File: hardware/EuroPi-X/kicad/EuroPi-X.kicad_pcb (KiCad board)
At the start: 2 copper layers, 86.5 x 109.2 mm, 154 parts, among them J1 Conn_01x16_Pin, J10 Thonkiconn_Mono_Jack, J11 Conn_02x08_Odd_Even, J12 Thonkiconn_Mono_Jack, J13 Thonkiconn_Mono_Jack, J14 Thonkiconn_Mono_Jack, J15 Thonkiconn_Mono_Jack, J16 Thonkiconn_Mono_Jack, J17 Thonkiconn_Mono_Jack, J18 Conn_01x30_Pin, J19 Conn_01x04_Pin, J2 Conn_01x16_Pin, J20 Conn_01x04_Pin, J21 Conn_01x04_Pin, J3 Thonkiconn_Mono_Jack, J4 Thonkiconn_Mono_Jack, J5 Conn_01x16_Pin, J6 Thonkiconn_Mono_Jack, J7 Thonkiconn_Mono_Jack, J8 Conn_01x16_Pin, J9 Thonkiconn_Mono_Jack, P1 USB_C_Plug_USB2.0, P2 Potentiometer_9mm_Vertical_Li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, P3 Potentiometer_9mm_Vertical_Li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, SW1 B1, SW2 B2, U1 LM4030-4.096, U10 MCP3428, U11 L7805, U2 LM4040DBZ-2.0, U3 LM4040DBZ-10, U4 RP2040, U7 TL074, U8 TL074, U9 MCP6004, Y1 Crystal_GND2

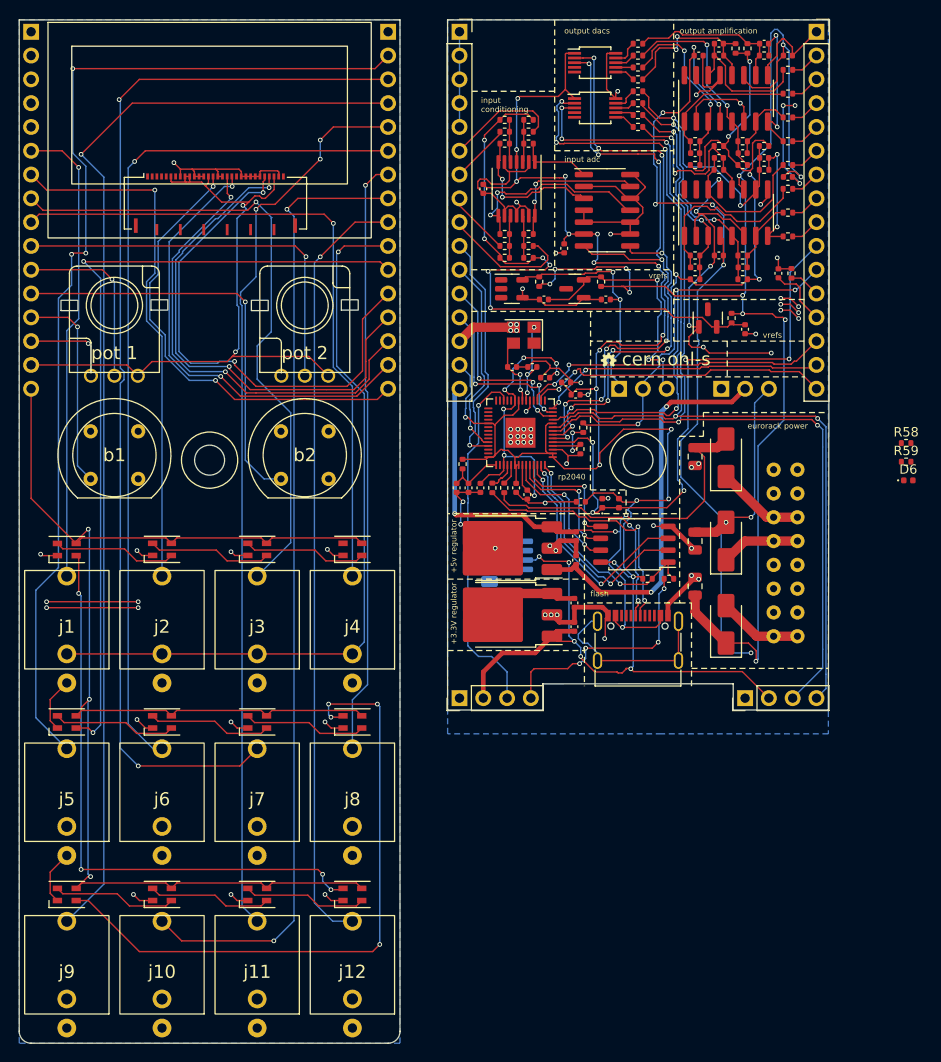
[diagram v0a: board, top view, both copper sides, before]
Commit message: save and export
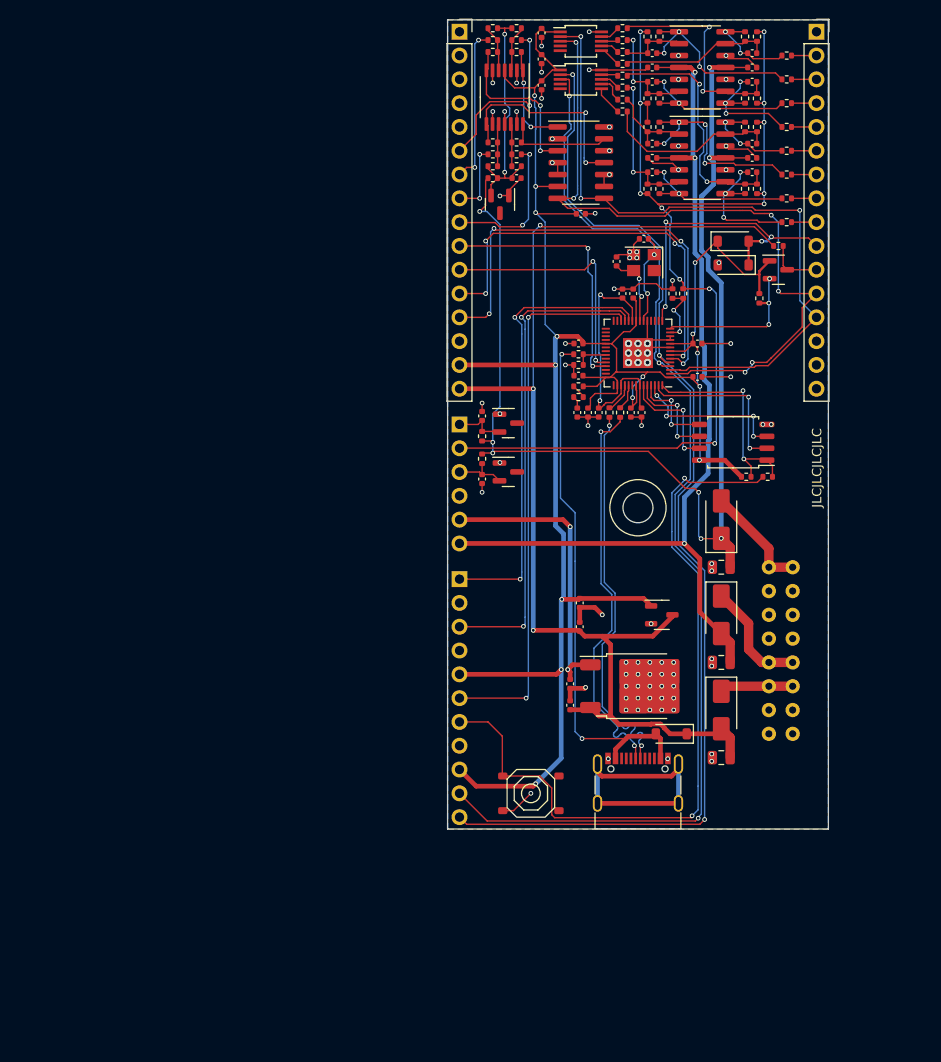
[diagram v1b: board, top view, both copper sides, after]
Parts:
- removed C18, C34: 100n, Capacitor_SMD:C_0402_1005Metric
- removed J1, J2: Conn_01x16_Pin, Connector_PinHeader_2.54mm:PinHeader_1x16_P2.54mm_Vertical
- removed J10, J12, J13, J14, J15, J16, J17, J3, J4, J6, J7, J9: Thonkiconn_Mono_Jack, Eurorack:Thonkiconn Mono Jack
- removed J18: Conn_01x30_Pin, Connector_FFC-FPC:Hirose_FH41-30S-0.5SH_1x30_1MP_1SH_P0.5mm_Horizontal
- removed J19, J21: Conn_01x04_Pin, Connector_PinHeader_2.54mm:PinHeader_1x04_P2.54mm_Vertical
- removed JUMPER1, JUMPER2: UNI/BIPOLAR, Connector_PinHeader_2.54mm:PinHeader_1x03_P2.54mm_Vertical
- removed LED1, LED10, LED11, LED12, LED2, LED3, LED4, LED5, LED6, LED7, LED8, LED9: SK6805, LED_SMD:LED_SK6805_PLCC4_2.4x2.7mm_P1.3mm
- removed P2, P3: Potentiometer_9mm_Vertical_Linear, Eurorack:Potentiometer 9mm Vertical Linear Centred
- removed R55: ~, Resistor_SMD:R_0402_1005Metric
- removed REF**: 128x64 SSD1306 OLED No Breakout, Eurorack:128x64 SSD1306 OLED No Breakout
- removed SW1: B1, Eurorack:Switch Tactile Momentary C&K
- removed SW2: B2, Eurorack:Switch Tactile Momentary C&K
- removed U1: LM4030-4.096, Package_TO_SOT_SMD:SOT-23-5
- added C37: 100n, Capacitor_SMD:C_0402_1005Metric, F.Cu at (55.8, 1.40)
- added C38: 100n, Capacitor_SMD:C_0402_1005Metric, F.Cu at (55.8, 4.19)
- added C39: 100n, Capacitor_SMD:C_0402_1005Metric, F.Cu at (72.4, 34.5)
- added C40: 100n, Capacitor_SMD:C_0402_1005Metric, F.Cu at (65.3, 41.9)
- added C41: 100n, Capacitor_SMD:C_0402_1005Metric, F.Cu at (64.4, 29.2)
- added J22: Conn_01x11_Pin, Connector_PinHeader_2.54mm:PinHeader_1x11_P2.54mm_Vertical, B.Cu at (47.0, 59.7)
- added Q1: BSS138, Package_TO_SOT_SMD:SOT-23, F.Cu at (81.0, 26.7)
- added R6: 10K, Resistor_SMD:R_0402_1005Metric, F.Cu at (79.0, 29.7)
- added R60: 200R, Resistor_SMD:R_0402_1005Metric, F.Cu at (59.7, 39.1)
- added R7: 10K, Resistor_SMD:R_0402_1005Metric, F.Cu at (81.0, 24.1)
- added SW3: ~, Eurorack:TS-1187A-B-A-B, F.Cu at (54.6, 82.5)
- added U12: LM4040DBZ-4.1, Package_TO_SOT_SMD:SOT-23, F.Cu at (52.2, 43.0)
- C1, C16: value 1u -> 100n
- C13, C17: value 100n -> 2u2
- C15: value 1u -> 2u2
- D3, D4, D6: footprint Diode_SMD:D_0402_1005Metric -> Diode_SMD:D_SOD-123
- J20: value Conn_01x04_Pin -> Conn_01x06_Pin; footprint Connector_JST:JST_SH_SM04B-SRSS-TB_1x04-1MP_P1.00mm_Horizontal -> Connector_PinHeader_2.54mm:PinHeader_1x06_P2.54mm_Vertical
- R24: value 27R4 -> 1R
- U11: footprint Package_TO_SOT_SMD:TO-252-3_TabPin2 -> Package_TO_SOT_SMD:TO-252-2
- U5: footprint Package_TO_SOT_SMD:TO-252-3_TabPin4 -> Package_TO_SOT_SMD:SOT-23-3
- U7, U8: footprint Package_SO:SOIC-16_3.9x9.9mm_P1.27mm -> Package_SO:SOIC-14_3.9x8.7mm_P1.27mm
- moved D6 37.0 mm to (69.6, 76.2), turned to 180 degrees
- moved R59 36.5 mm to (59.7, 36.8)
- moved R58 36.2 mm to (59.7, 35.7), turned to 180 degrees
- moved C28 32.3 mm to (74.9, 78.7), turned to 180 degrees
- moved D3 30.5 mm to (76.2, 23.6), turned to 0 degrees
- moved R3 29.5 mm to (50.5, 16.9), turned to 180 degrees
- moved C4 29.2 mm to (53.1, 16.9), turned to 0 degrees
- moved D4 29.0 mm to (76.2, 26.2), turned to 180 degrees
- moved D5 26.9 mm to (74.9, 73.7), turned to -90 degrees
- moved U3 25.3 mm to (51.3, 19.7), turned to -90 degrees
- moved C6 24.3 mm to (65.5, 29.2), turned to 90 degrees
- moved R2 22.8 mm to (49.4, 46.8), turned to 90 degrees
- moved U2 20.8 mm to (52.2, 48.2), turned to 0 degrees
- moved U11 20.5 mm to (66.0, 71.1), turned to 0 degrees
- moved C3 20.3 mm to (49.4, 49.0), turned to -90 degrees
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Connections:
- net QSPI_CS renamed /QSPI_CS
- net QSPI_SCLK renamed /QSPI_SCLK
- net QSPI_SD0 renamed /QSPI_SD0
- net QSPI_SD1 renamed /QSPI_SD1
- net QSPI_SD2 renamed /QSPI_SD2
- net QSPI_SD3 renamed /QSPI_SD3
- net USB_DN renamed /USB_DN
- net USB_DP renamed /USB_DP
- net XTAL_IN renamed /XTAL_IN
- net XTAL_OUT renamed /XTAL_OUT
- C1 pad 1: Net-(U4-VREG_VOUT) -> +3.3V
- C10 pad 1: IOVDD -> +3.3V
- C11 pad 1: Net-(U7D-+) -> Net-(U7D--)
- C12 pad 1: Net-(U8D-+) -> Net-(U8D--)
- C13 pad 1: ADC_AVDD -> +1V1
- C14 pad 1: IOVDD -> +3.3V
- C15 pad 1: ADC_AVDD -> +3.3V
- C16 pad 1: IOVDD -> +1V1
- C17 pad 1: IOVDD -> /ADC_ADVDD
- C19 pad 1: Net-(U7A-+) -> Net-(U7A--)
- C20 pad 1: Net-(U8A-+) -> Net-(U8A--)
- C27 pad 1: IOVDD -> +3.3V
- C29 pad 1: Net-(U7B-+) -> Net-(U7B--)
- C30 pad 1: Net-(U8B-+) -> Net-(U8B--)
- C31 pad 1: IOVDD -> +3.3V
- C32 pad 1: Net-(U7C-+) -> Net-(U7C--)
- C33 pad 1: Net-(U8C-+) -> Net-(U8C--)
- C5 pad 1: Net-(U4-VREG_VOUT) -> +3.3V
- C6 pad 1: Net-(U4-VREG_VOUT) -> +3.3V
- D3 pad 1: IOVDD -> +3.3V
- DAC1 pad 1: IOVDD -> +3.3V
- DAC2 pad 1: IOVDD -> +3.3V
- J20 pad 1: Earth -> /-4.096VREF
- J20 pad 2: IOVDD -> /DAC_OFFSET
- J20 pad 3: /I2C1_SDA -> /-2.048VREF
- J20 pad 4: /I2C1_SCL -> unconnected-(J20-Pin_4-Pad4)
- J5 pad 15: IOVDD -> +3.3V
- J8 pad 11: /NEOPIXEL_DATA -> /NEOPIXEL_DATA_5V
- J8 pad 12: /IREF -> /I2C0_SDA
- J8 pad 13: /VCOMH -> /I2C0_SCL
- J8 pad 14: /OLED_CLK -> Earth
- J8 pad 15: /OLED_DIN -> Earth
- J8 pad 16: /OLED_D/C -> Earth
- R10 pad 1: IOVDD -> +3.3V
- R12 pad 1: Net-(U7D-+) -> Net-(U7D--)
- R13 pad 1: Net-(U7D-+) -> Net-(U7D--)
- R14 pad 1: Net-(U8D-+) -> Net-(U8D--)
- R15 pad 1: Net-(U8D-+) -> Net-(U8D--)
- R16 pad 2: Net-(U7D-+) -> Net-(U7D--)
- R17 pad 2: Net-(U8D-+) -> Net-(U8D--)
- R24 pad 1: IOVDD -> /ADC_ADVDD
- R24 pad 2: ADC_AVDD -> /ADC_VREF
- R27 pad 1: Net-(U7A-+) -> Net-(U7A--)
- R28 pad 1: Net-(U7A-+) -> Net-(U7A--)
- R29 pad 1: Net-(U8A-+) -> Net-(U8A--)
- R30 pad 1: Net-(U8A-+) -> Net-(U8A--)
- R31 pad 2: Net-(U7A-+) -> Net-(U7A--)
- R32 pad 2: Net-(U8A-+) -> Net-(U8A--)
- R41 pad 1: Net-(U7B-+) -> Net-(U7B--)
- R42 pad 1: Net-(U7B-+) -> Net-(U7B--)
- R43 pad 1: Net-(U8B-+) -> Net-(U8B--)
- R44 pad 1: Net-(U8B-+) -> Net-(U8B--)
- R45 pad 2: Net-(U7B-+) -> Net-(U7B--)
- R46 pad 2: Net-(U8B-+) -> Net-(U8B--)
- R49 pad 1: Net-(U7C-+) -> Net-(U7C--)
- R50 pad 1: Net-(U7C-+) -> Net-(U7C--)
- R51 pad 1: Net-(U8C-+) -> Net-(U8C--)
- R52 pad 1: Net-(U8C-+) -> Net-(U8C--)
- R53 pad 2: Net-(U7C-+) -> Net-(U7C--)
- R54 pad 2: Net-(U8C-+) -> Net-(U8C--)
- U10 pad 6: IOVDD -> +3.3V
- U4 pad 1: IOVDD -> +3.3V
- U4 pad 10: IOVDD -> +3.3V
- U4 pad 11: /NEOPIXEL_DATA -> Earth
- U4 pad 12: /BUTTON_2 -> Earth
- U4 pad 13: /BUTTON_1 -> /OUTPUT_MODE
- U4 pad 14: /OLED_DIN -> /NEOPIXEL_DATA_3V3
- U4 pad 15: unconnected-(U4-GPIO12-Pad15) -> /INPUT_DETECT
- U4 pad 16: /OLED_D/C -> unconnected-(U4-GPIO13-Pad16)
- U4 pad 17: /OLED_CLK -> unconnected-(U4-GPIO14-Pad17)
- U4 pad 2: IOVDD -> /I2C0_SDA
- U4 pad 22: IOVDD -> +3.3V
- U4 pad 23: Net-(U4-VREG_VOUT) -> +1V1
- U4 pad 24: SWCLK -> /SWCLK
- U4 pad 25: SWDIO -> /SWDIO
- U4 pad 3: Earth -> /I2C0_SCL
- U4 pad 33: IOVDD -> +3.3V
- U4 pad 36: unconnected-(U4-GPIO24-Pad36) -> /USB_DETECT
- U4 pad 4: /OUTPUT_MODE -> /I2C1_SDA
- U4 pad 42: IOVDD -> +3.3V
- U4 pad 43: ADC_AVDD -> /ADC_VDD
- U4 pad 44: VREG_IN -> +3.3V
- U4 pad 45: Net-(U4-VREG_VOUT) -> +1V1
- U4 pad 48: IOVDD -> /USB_VDD
- U4 pad 49: IOVDD -> +3.3V
- U4 pad 5: /INPUT_DETECT -> /I2C1_SCL
- U4 pad 50: Net-(U4-VREG_VOUT) -> +1V1
- U4 pad 6: /I2C0_SDA -> /BUTTON_1
- U4 pad 7: /I2C0_SCL -> /BUTTON_2
- U4 pad 8: /I2C1_SDA -> +3.3V
- U4 pad 9: /I2C1_SCL -> Earth
- U5 pad 1: IOVDD -> +3.3V
- U6 pad 8: IOVDD -> +3.3V
- U7 pad 10: Net-(U7C-+) -> Earth
- U7 pad 12: Net-(U7D-+) -> Earth
- U7 pad 13: Earth -> Net-(U7D--)
- U7 pad 2: Earth -> Net-(U7A--)
- U7 pad 3: Net-(U7A-+) -> Earth
- U7 pad 5: Net-(U7B-+) -> Earth
- U7 pad 6: Earth -> Net-(U7B--)
- U7 pad 9: Earth -> Net-(U7C--)
- U8 pad 10: Net-(U8C-+) -> Earth
- U8 pad 12: Net-(U8D-+) -> Earth
- U8 pad 13: Earth -> Net-(U8D--)
- U8 pad 2: Earth -> Net-(U8A--)
- U8 pad 3: Net-(U8A-+) -> Earth
- U8 pad 5: Net-(U8B-+) -> Earth
- U8 pad 6: Earth -> Net-(U8B--)
- U8 pad 9: Earth -> Net-(U8C--)
- U9 pad 4: IOVDD -> +3.3V
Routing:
- net IOVDD: track 234.5 -> 0.00 mm, vias 23 -> 0
- net +3.3V: track 0.00 -> 231.7 mm, vias 0 -> 15
- net /+5V_FRONT: track 157.2 -> 0.00 mm, vias 3 -> 0
- net Earth: track 230.8 -> 86.7 mm, vias 62 -> 90
- net /CV_OUTPUT_3_FRONT: track 119.5 -> 0.00 mm, vias 1 -> 0
- net /CV_OUTPUT_2_FRONT: track 115.3 -> 0.00 mm, vias 2 -> 0
- net /CV_OUTPUT_1_FRONT: track 111.8 -> 0.00 mm, vias 3 -> 0
- net /CV_OUTPUT_7_FRONT: track 103.4 -> 0.00 mm, vias 2 -> 0
- net /CV_OUTPUT_4_FRONT: track 96.3 -> 0.00 mm, vias 3 -> 0
- net /CV_OUTPUT_5_FRONT: track 92.5 -> 0.00 mm, vias 1 -> 0
- net /NEOPIXEL_DATA_FRONT: track 86.2 -> 0.00 mm, vias 2 -> 0
- net /CV_OUTPUT_8_FRONT: track 82.8 -> 0.00 mm, vias 1 -> 0
- net /INPUT_DETECT_FRONT: track 80.8 -> 0.00 mm, vias 1 -> 0
- net /GND_FRONT: track 78.8 -> 0.00 mm, vias 16 -> 0
- net /CV_INPUT_4_FRONT: track 71.5 -> 0.00 mm, vias 1 -> 0
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- removed copper zone on B.Cu, net /GND_FRONT
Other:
- board size 86.5 x 109.2 mm -> 40.6 x 86.4 mm
- board text added: "+3.3V"
- board text added: "5V rail"
- board text added: "JLCJLCJLCJLC"
- board text added: "bootsel"
- board text added: "gnd"
- board text added: "no 5V rail"
- board text added: "run"
- board text added: "scl"
- board text added: "sda"
- board text added: "swclk"
- board text added: "swdio"
- board text added: "version 1.0"
- board text removed: "+3.3V regulator"
- board text removed: "+5v regulator"
- board text removed: "b1"
- board text removed: "b2"
- board text removed: "eurorack power"
- board text removed: "expand"
- board text removed: "flash"
- board text removed: "input adc"
- board text removed: "input conditioning"
- board text removed: "internal +5V"
- board text removed: "i²c"
- board text removed: "j1"
- board text removed: "j10"
- board text removed: "j11"
- board text removed: "j12"
- board text removed: "j2"
- board text removed: "j3"
- board text removed: "j4"
- board text removed: "j5"
- board text removed: "j6"
- board text removed: "j7"
- board text removed: "j8"
- board text removed: "j9"
- board text removed: "output amplification"
- board text removed: "output dacs"
- board text removed: "pot 1"
- board text removed: "pot 2"
- board text removed: "rp2040"
- board text removed: "vrefs"

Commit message: undelete board side
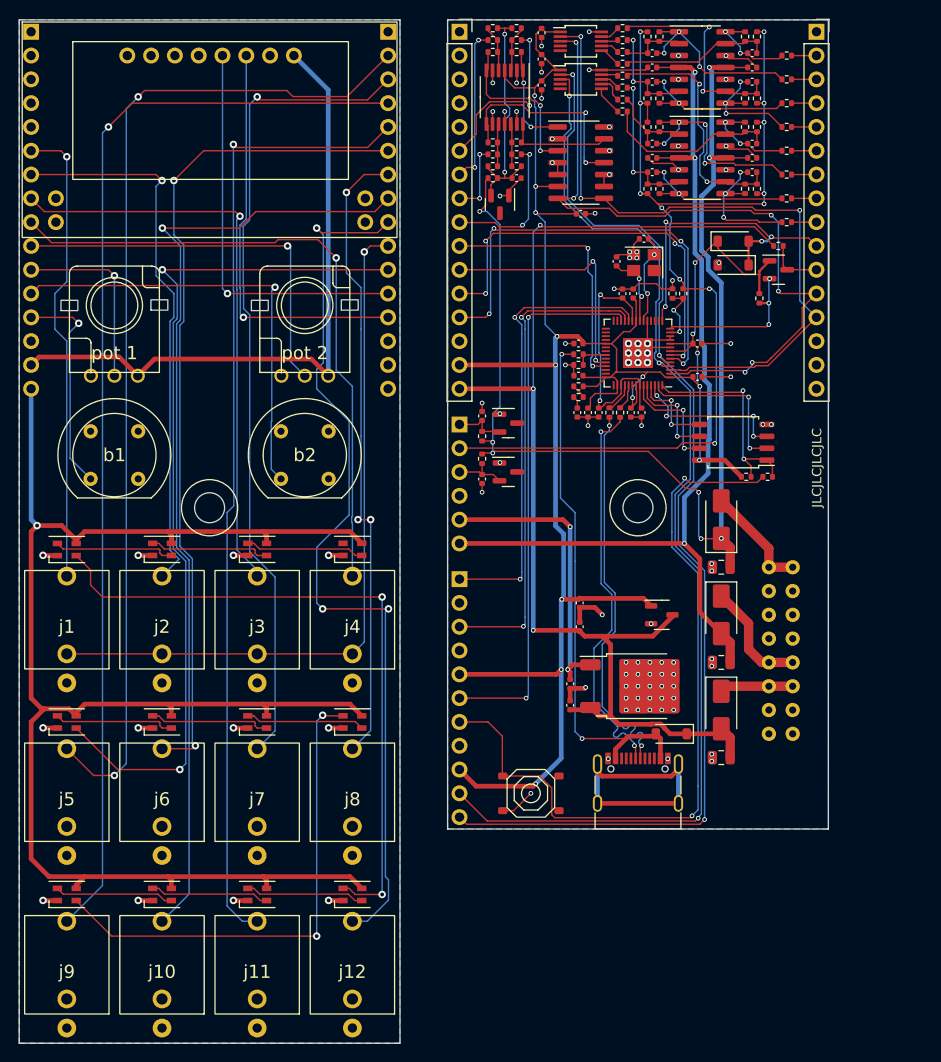
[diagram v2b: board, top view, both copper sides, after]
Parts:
- added J1: Conn_01x16_Pin, Connector_PinHeader_2.54mm:PinHeader_1x16_P2.54mm_Vertical, B.Cu at (1.27, 1.27)
- added J10: Thonkiconn_Mono_Jack, Eurorack:Thonkiconn Mono Jack, F.Cu at (15.2, 64.8)
- added J12: Thonkiconn_Mono_Jack, Eurorack:Thonkiconn Mono Jack, F.Cu at (25.4, 83.2)
- added J13: Thonkiconn_Mono_Jack, Eurorack:Thonkiconn Mono Jack, F.Cu at (35.6, 83.2)
- added J14: Thonkiconn_Mono_Jack, Eurorack:Thonkiconn Mono Jack, F.Cu at (5.08, 101.6)
- added J15: Thonkiconn_Mono_Jack, Eurorack:Thonkiconn Mono Jack, F.Cu at (15.2, 101.6)
- added J16: Thonkiconn_Mono_Jack, Eurorack:Thonkiconn Mono Jack, F.Cu at (25.4, 101.6)
- added J17: Thonkiconn_Mono_Jack, Eurorack:Thonkiconn Mono Jack, F.Cu at (35.6, 101.6)
- added J2: Conn_01x16_Pin, Connector_PinHeader_2.54mm:PinHeader_1x16_P2.54mm_Vertical, B.Cu at (39.4, 1.27)
- added J3: Thonkiconn_Mono_Jack, Eurorack:Thonkiconn Mono Jack, F.Cu at (5.08, 64.8)
- added J4: Thonkiconn_Mono_Jack, Eurorack:Thonkiconn Mono Jack, F.Cu at (25.4, 64.8)
- added J6: Thonkiconn_Mono_Jack, Eurorack:Thonkiconn Mono Jack, F.Cu at (5.08, 83.2)
- added J7: Thonkiconn_Mono_Jack, Eurorack:Thonkiconn Mono Jack, F.Cu at (15.2, 83.2)
- added J9: Thonkiconn_Mono_Jack, Eurorack:Thonkiconn Mono Jack, F.Cu at (35.6, 64.8)
- added LED1: SK6805, LED_SMD:LED_SK6805_PLCC4_2.4x2.7mm_P1.3mm, F.Cu at (5.08, 74.9)
- added LED10: SK6805, LED_SMD:LED_SK6805_PLCC4_2.4x2.7mm_P1.3mm, F.Cu at (25.4, 56.5)
- added LED11: SK6805, LED_SMD:LED_SK6805_PLCC4_2.4x2.7mm_P1.3mm, F.Cu at (15.2, 56.5)
- added LED12: SK6805, LED_SMD:LED_SK6805_PLCC4_2.4x2.7mm_P1.3mm, F.Cu at (35.6, 56.5)
- added LED2: SK6805, LED_SMD:LED_SK6805_PLCC4_2.4x2.7mm_P1.3mm, F.Cu at (5.08, 93.3)
- added LED3: SK6805, LED_SMD:LED_SK6805_PLCC4_2.4x2.7mm_P1.3mm, F.Cu at (15.2, 74.9)
- added LED4: SK6805, LED_SMD:LED_SK6805_PLCC4_2.4x2.7mm_P1.3mm, F.Cu at (15.2, 93.3)
- added LED5: SK6805, LED_SMD:LED_SK6805_PLCC4_2.4x2.7mm_P1.3mm, F.Cu at (25.4, 74.9)
- added LED6: SK6805, LED_SMD:LED_SK6805_PLCC4_2.4x2.7mm_P1.3mm, F.Cu at (25.4, 93.3)
- added LED7: SK6805, LED_SMD:LED_SK6805_PLCC4_2.4x2.7mm_P1.3mm, F.Cu at (35.6, 74.9)
- added LED8: SK6805, LED_SMD:LED_SK6805_PLCC4_2.4x2.7mm_P1.3mm, F.Cu at (35.6, 93.3)
- added LED9: SK6805, LED_SMD:LED_SK6805_PLCC4_2.4x2.7mm_P1.3mm, F.Cu at (5.08, 56.5)
- added OLED1: ~, Eurorack:Enoki OLED SSD1306 128x64, F.Cu at (11.5, 3.81)
- added P2: Potentiometer_9mm_Vertical_Linear, Eurorack:Potentiometer 9mm Vertical Linear Centred, F.Cu at (10.2, 30.5)
- added P3: Potentiometer_9mm_Vertical_Linear, Eurorack:Potentiometer 9mm Vertical Linear Centred, F.Cu at (30.5, 30.5)
- added SW1: B1, Eurorack:Switch Tactile Momentary C&K, F.Cu at (7.62, 49.0)
- added SW2: B2, Eurorack:Switch Tactile Momentary C&K, F.Cu at (27.9, 49.0)
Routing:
- net /+5V_FRONT: track 0.00 -> 170.7 mm, vias 0 -> 1
- net /CV_OUTPUT_3_FRONT: track 0.00 -> 117.5 mm, vias 0 -> 1
- net /CV_OUTPUT_1_FRONT: track 0.00 -> 108.8 mm, vias 0 -> 2
- net /CV_OUTPUT_4_FRONT: track 0.00 -> 103.0 mm, vias 0 -> 1
- net /CV_OUTPUT_7_FRONT: track 0.00 -> 102.1 mm, vias 0 -> 1
- net /CV_OUTPUT_8_FRONT: track 0.00 -> 95.8 mm, vias 0 -> 3
- net /NEOPIXEL_DATA_FRONT: track 0.00 -> 92.0 mm, vias 0 -> 2
- net /CV_OUTPUT_5_FRONT: track 0.00 -> 89.5 mm, vias 0 -> 2
- net /CV_OUTPUT_2_FRONT: track 0.00 -> 87.6 mm, vias 0 -> 1
- net /INPUT_DETECT_FRONT: track 0.00 -> 76.7 mm, vias 0 -> 1
- net Net-(LED8-DOUT): track 0.00 -> 71.6 mm, vias 0 -> 2
- net /+3.3V_FRONT: track 0.00 -> 70.1 mm
- net /CV_INPUT_4_FRONT: track 0.00 -> 69.2 mm, vias 0 -> 1
- net /CV_OUTPUT_6_FRONT: track 0.00 -> 67.5 mm, vias 0 -> 3
- net /CV_INPUT_3_FRONT: track 0.00 -> 62.5 mm, vias 0 -> 1
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- added copper zone on B.Cu, net /GND_FRONT
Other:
- board size 40.6 x 86.4 mm -> 86.4 x 109.2 mm
- board text added: "b1"
- board text added: "b2"
- board text added: "j1"
- board text added: "j10"
- board text added: "j11"
- board text added: "j12"
- board text added: "j2"
- board text added: "j3"
- board text added: "j4"
- board text added: "j5"
- board text added: "j6"
- board text added: "j7"
- board text added: "j8"
- board text added: "j9"
- board text added: "pot 1"
- board text added: "pot 2"
